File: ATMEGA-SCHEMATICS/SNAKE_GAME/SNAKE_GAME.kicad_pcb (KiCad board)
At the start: 2 copper layers, 136.8 x 95.5 mm, 40 parts, among them J1 GRID, J10 VCC, J11 PJ-102A, J3 Conn_01x03_Pin, J4 USB_ASP, J5 BUTTONS, J6 JOYSTICK, J7 UART_TERM, J8 PCF_SCREEN, J9 GROUND, SW1 SW_Push, U1 ATmega168A-P, Y1 Crystal

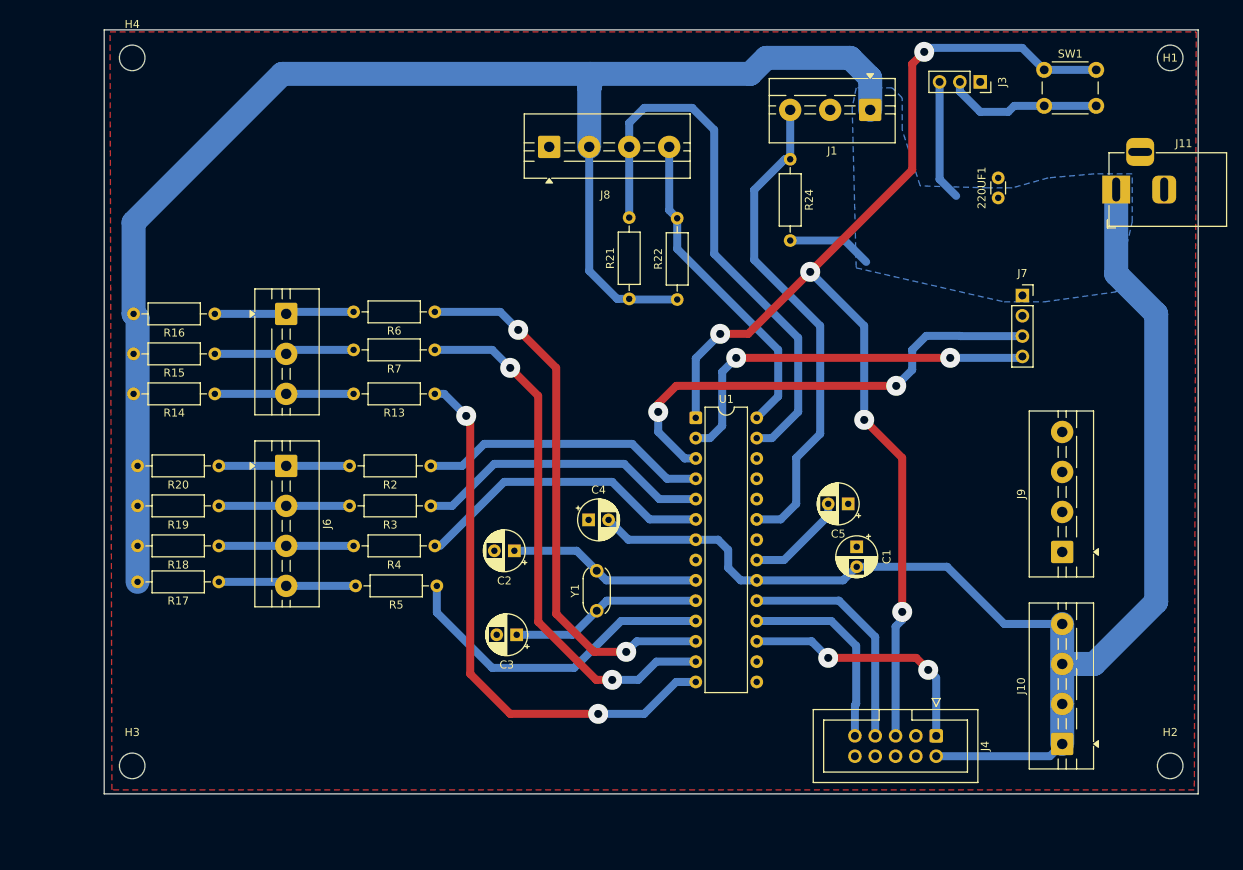
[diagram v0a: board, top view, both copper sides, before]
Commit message: .
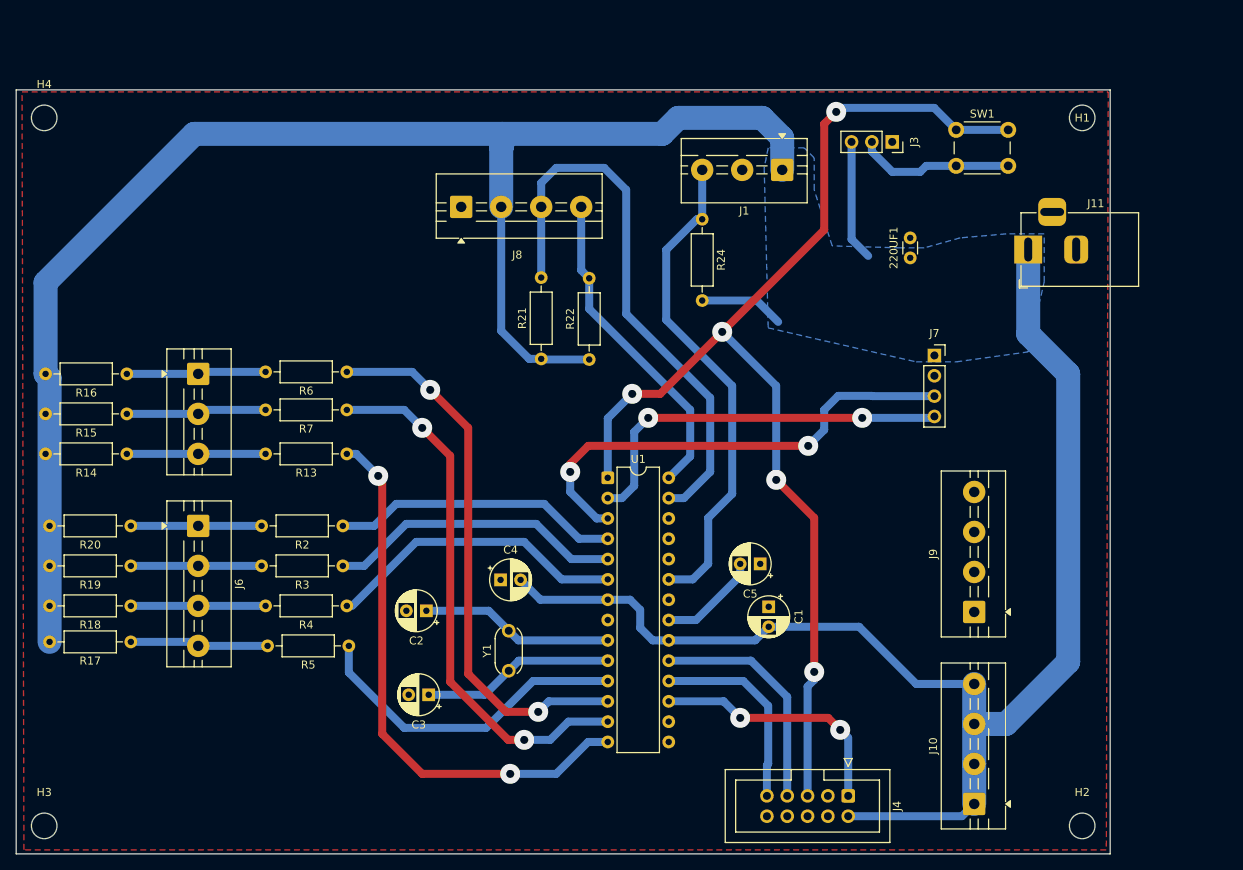
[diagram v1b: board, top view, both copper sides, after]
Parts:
- moved J9 13.3 mm to (121.0, -30.0)
- moved 220UF1 13.3 mm to (113.0, -74.2)
- moved C1 13.3 mm to (95.3, -30.6)
- moved C2 13.3 mm to (52.5, -30.1)
- moved C3 13.3 mm to (52.8, -19.6)
- moved C4 13.3 mm to (61.8, -34.0)
- moved C5 13.3 mm to (94.2, -36.0)
- moved H1 13.3 mm to (134.5, -91.8)
- moved H2 13.3 mm to (134.5, -3.25)
- moved H3 13.3 mm to (4.75, -3.25)
- moved H4 13.3 mm to (4.75, -91.8)
- moved J1 13.3 mm to (97.0, -85.2)
- moved J10 13.3 mm to (121.0, -5.99)
- moved J11 13.3 mm to (127.8, -75.3)
- moved J3 13.3 mm to (110.8, -88.8)
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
